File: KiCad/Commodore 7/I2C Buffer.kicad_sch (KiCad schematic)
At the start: 2 parts, among them U6 TCA9509DGKR

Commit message: uhhhhhhhh idk
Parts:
- U6: footprint DGK8 -> TCA9509DGKR:DGK8
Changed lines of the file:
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@@
 			)
 		)
-		(property "Footprint" "DGK8"
+		(property "Footprint" "TCA9509DGKR:DGK8"
 			(at 120.65 95.25 0)
 			(effects

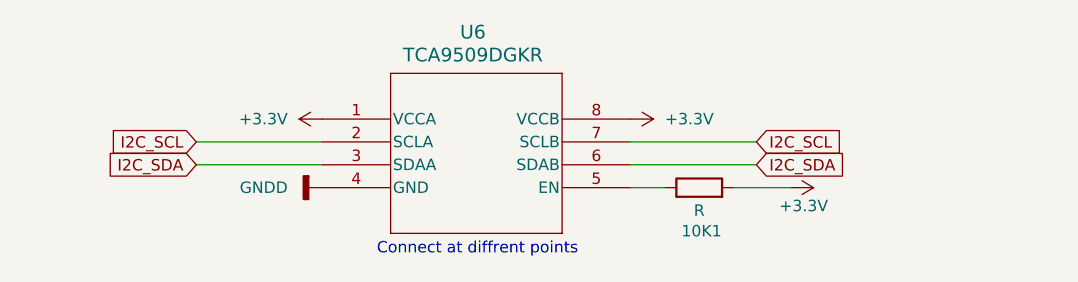
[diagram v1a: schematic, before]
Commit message: i sitll got mroe to do ssry yall
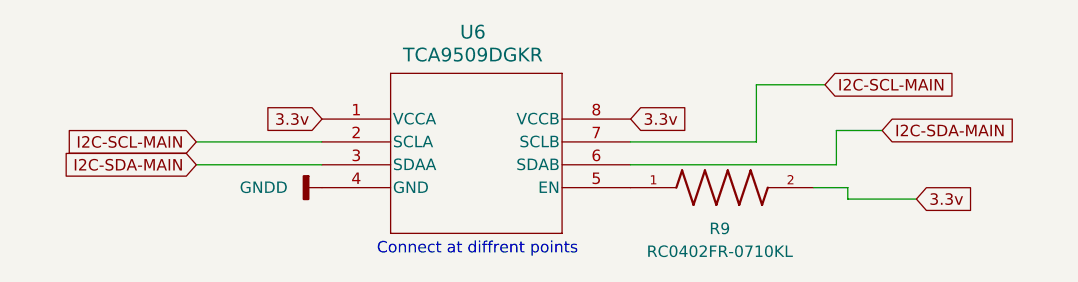
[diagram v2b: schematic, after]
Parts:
- removed 10K1: R, symbol Device:R
- added R9: RC0402FR-0710KL, RC0402FR:YAG_R0402_YAG, symbol RC0402FR-0710KL:RC0402FR-0710KL
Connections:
- net at U6.5 (EN): now also R9.1
- net +3.3V renamed 3.3v
- net 3.3v: now also R9.2
- net I2C_SCL renamed I2C-SCL-MAIN
- net I2C_SDA renamed I2C-SDA-MAIN
